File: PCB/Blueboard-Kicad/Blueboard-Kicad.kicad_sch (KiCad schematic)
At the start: 218 parts, among them SW1 M1, SW10 SHIFT, SW100 NM5, SW101 NM2, SW102 *, SW103 NM9, SW104 NM6, SW105 NM3, SW106 ., SW107 -, SW108 +, SW11 CTL, SW110 Enter, SW12 1, SW13 Q, SW14 A, SW15 Z, SW16 WIN, SW17 F1, SW18 2, SW19 W, SW2 ESC, SW20 S, SW21 X, SW22 ALT, SW23 F2, SW24 3, SW25 E, SW26 D, SW27 C, SW28 F3, SW29 4, SW3 M1, SW30 R, SW31 F, SW32 V, SW33 F4, SW34 5, SW35 T, SW36 G, SW37 B, SW38 SPACE, SW39 6, SW4 M1, SW40 Y, SW41 H, SW42 N, SW43 7, SW44 U, SW45 J, SW46 M, SW47 F5, SW48 F6, SW49 8, SW5 M1, SW50 I, SW51 K, SW52 <, SW53 ALT, SW54 F7, SW55 9, SW56 O, SW57 L, SW58 >, SW59 WIN, SW6 M1, SW60 F8, SW61 0, SW62 P, SW63 ;, SW64 ?, SW65 Menu, SW66 +, SW67 -, SW68 {, SW69 @, SW7 TILDA, SW70 SHIFT, SW71 CTR, SW72 }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

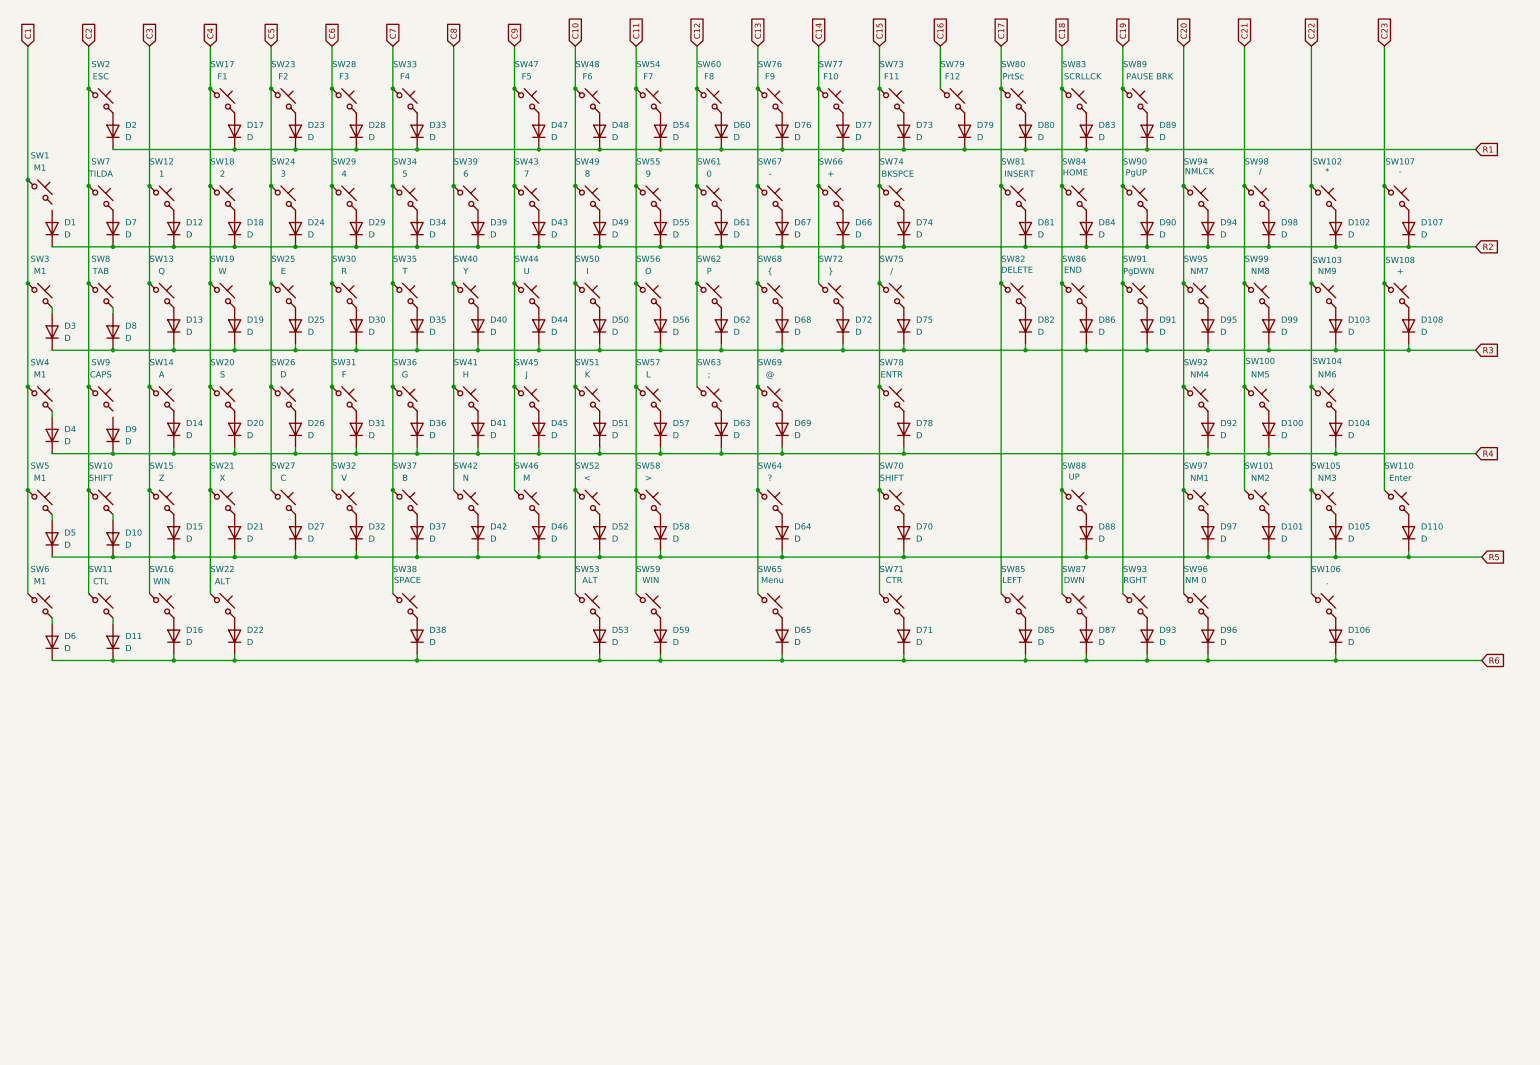
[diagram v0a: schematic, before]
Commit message: Finished Schematc + Layedout Components
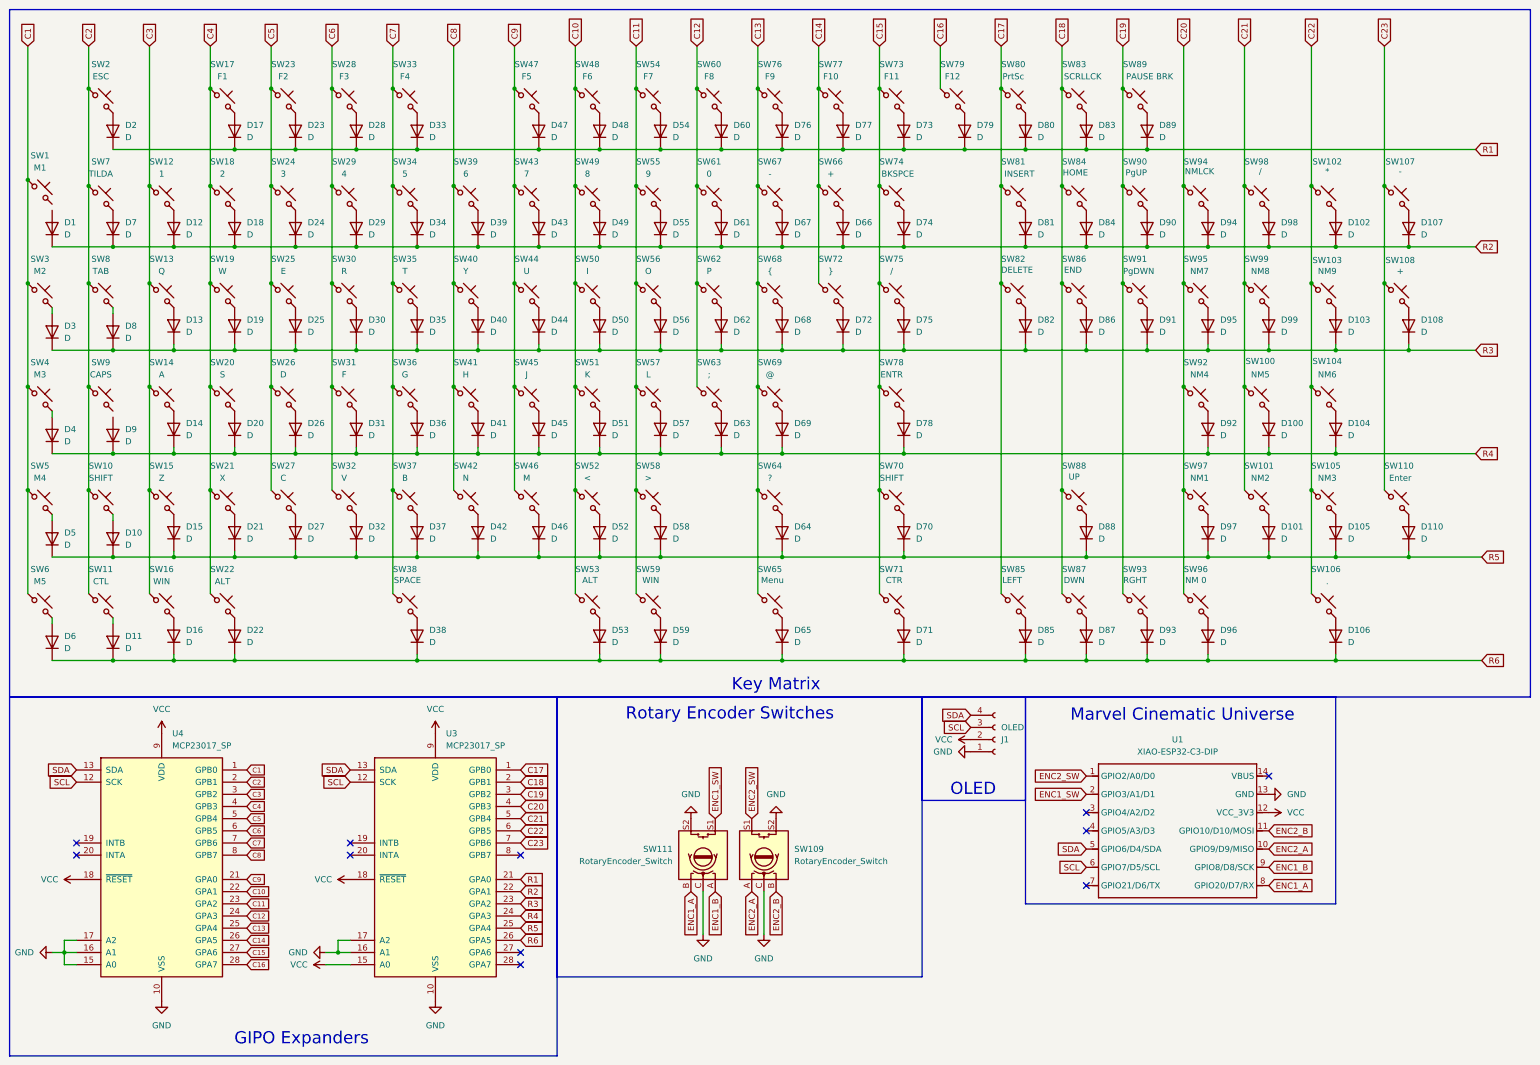
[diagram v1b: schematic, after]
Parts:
- added J1: OLED, KiCad-SSD1306-0.91-OLED-4pin-128x32:SSD1306-0.91-OLED-4pin-128x32, symbol Connector:Conn_01x04_Socket
- added SW109, SW111: RotaryEncoder_Switch, Rotary_Encoder:RotaryEncoder_Alps_EC11E-Switch_Vertical_H20mm_MountingHoles, symbol Device:RotaryEncoder_Switch
- added U1: XIAO-ESP32-C3-DIP, Seeed Studio XIAO Series Library:XIAO-ESP32C3-DIP, symbol Seeed_Studio_XIAO_Series:XIAO-ESP32-C3-DIP
- added U3, U4: MCP23017_SP, Package_DIP:DIP-28_W7.62mm, symbol Interface_Expansion:MCP23017_SP
- D1, D10, D100, D101, D102, D103, D104, D105, D106, D107, D108, D11, D110, D12, D13, D14, D15, D16, D17, D18, D19, D2, D20, D21, D22, D23, D24, D25, D26, D27, D28, D29, D3, D30, D31, D32, D33, D34, D35, D36, D37, D38, D39, D4, D40, D41, D42, D43, D44, D45, D46, D47, D48, D49, D5, D50, D51, D52, D53, D54, D55, D56, D57, D58, D59, D6, D60, D61, D62, D63, D64, D65, D66, D67, D68, D69, D7, D70, D71, D72, D73, D74, D75, D76, D77, D78, D79, D8, D80, D81, D82, D83, D84, D85, D86, D87, D88, D89, D9, D90, D91, D92, D93, D94, D95, D96, D97, D98, D99: footprint (none) -> Diode_THT:D_DO-41_SOD81_P7.62mm_Horizontal
- SW1, SW100, SW101, SW102, SW103, SW104, SW105, SW106, SW107, SW12, SW13, SW14, SW15, SW17, SW18, SW19, SW2, SW20, SW21, SW23, SW24, SW25, SW26, SW27, SW28, SW29, SW30, SW31, SW32, SW33, SW34, SW35, SW36, SW37, SW39, SW40, SW41, SW42, SW43, SW44, SW45, SW46, SW47, SW48, SW49, SW50, SW51, SW52, SW54, SW55, SW56, SW57, SW58, SW60, SW61, SW62, SW63, SW64, SW66, SW67, SW68, SW69, SW7, SW76, SW77, SW79, SW80, SW81, SW82, SW83, SW84, SW85, SW86, SW87, SW88, SW89, SW90, SW91, SW92, SW93, SW94, SW95, SW97, SW98, SW99: footprint (none) -> Keyboard:SW_Cherry_MX1A_1.00u_PCB
- SW10, SW78: footprint (none) -> Keyboard:SW_Cherry_MX1A_2.25u_PCB
- SW108, SW110: footprint (none) -> Keyboard:SW_Cherry_MX1A_2.00u_Vertical_PCB
- SW11, SW16, SW22, SW53, SW59, SW65, SW71, SW72, SW73: footprint (none) -> Keyboard:SW_Cherry_MX1A_1.25u_PCB
- SW3: value M1 -> M2; footprint (none) -> Keyboard:SW_Cherry_MX1A_1.00u_PCB
- SW38: footprint (none) -> Keyboard:SW_Cherry_MX1A_6.25u_PCB
- SW4: value M1 -> M3; footprint (none) -> Keyboard:SW_Cherry_MX1A_1.00u_PCB
- SW5: value M1 -> M4; footprint (none) -> Keyboard:SW_Cherry_MX1A_1.00u_PCB
- SW6: value M1 -> M5; footprint (none) -> Keyboard:SW_Cherry_MX1A_1.00u_PCB
- SW70: footprint (none) -> Keyboard:SW_Cherry_MX1A_2.75u_PCB
- SW74, SW96: footprint (none) -> Keyboard:SW_Cherry_MX1A_2.00u_PCB
- SW75, SW8: footprint (none) -> Keyboard:SW_Cherry_MX1A_1.50u_PCB
- SW9: footprint (none) -> Keyboard:SW_Cherry_MX1A_1.75u_PCB
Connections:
- net C1: now also U4.1 (GPB0)
- net C10: now also U4.22 (GPA1)
- net C11: now also U4.23 (GPA2)
- net C12: now also U4.24 (GPA3)
- net C13: now also U4.25 (GPA4)
- net C14: now also U4.26 (GPA5)
- net C15: now also U4.27 (GPA6)
- net C16: now also U4.28 (GPA7)
- net C17: now also U3.1 (GPB0)
- net C18: now also U3.2 (GPB1)
- net C19: now also U3.3 (GPB2)
- net C2: now also U4.2 (GPB1)
- net C20: now also U3.4 (GPB3)
- net C21: now also U3.5 (GPB4)
- net C22: now also U3.6 (GPB5)
- net C23: now also U3.7 (GPB6)
- net C3: now also U4.3 (GPB2)
- net C4: now also U4.4 (GPB3)
- net C5: now also U4.5 (GPB4)
- net C6: now also U4.6 (GPB5)
- net C7: now also U4.7 (GPB6)
- net C8: now also U4.8 (GPB7)
- net C9: now also U4.21 (GPA0)
- net R1: now also U3.21 (GPA0)
- net R2: now also U3.22 (GPA1)
- net R3: now also U3.23 (GPA2)
- net R4: now also U3.24 (GPA3)
- net R5: now also U3.25 (GPA4)
- net R6: now also U3.26 (GPA5)
- new net ENC1_A: SW111.B, U1.8 (GPIO20/D7/RX)
- new net ENC1_B: SW111.A, U1.9 (GPIO8/D8/SCK)
- new net ENC1_SW: SW111.S1, U1.2 (GPIO3/A1/D1)
- new net ENC2_A: SW109.A, U1.10 (GPIO9/D9/MISO)
- new net ENC2_B: SW109.B, U1.11 (GPIO10/D10/MOSI)
- new net ENC2_SW: SW109.S1, U1.1 (GPIO2/A0/D0)
- new net GND: J1.1 (Pin_1), SW109.C, SW109.S2, SW111.C, SW111.S2, U1.13 (GND), U3.10 (VSS), U3.16 (A1), U3.17 (A2), U4.10 (VSS), U4.15 (A0), U4.16 (A1), U4.17 (A2)
- new net SCL: J1.3 (Pin_3), U1.6 (GPIO7/D5/SCL), U3.12 (SCK), U4.12 (SCK)
- new net SDA: J1.4 (Pin_4), U1.5 (GPIO6/D4/SDA), U3.13 (SDA), U4.13 (SDA)
- new net VCC: J1.2 (Pin_2), U1.12 (VCC_3V3), U3.15 (A0), U3.18 (~{RESET}), U3.9 (VDD), U4.18 (~{RESET}), U4.9 (VDD)
- no-connect marks 0 -> 11
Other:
- note added: "GIPO Expanders"
- note added: "Key Matrix"
- note added: "Marvel Cinematic Universe"
- note added: "OLED"
- note added: "Rotary Encoder Switches"
